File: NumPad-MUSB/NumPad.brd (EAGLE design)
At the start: 85.1 x 137.2 mm, 149 parts, among them J1 J, J10 J, J11 J, J12 J, J13 J, J14 J, J15 J, J16 J, J17 J, J2 J, J3 J, J4 J, J5 J, J6 J, J7 J, J8 J, J9 J

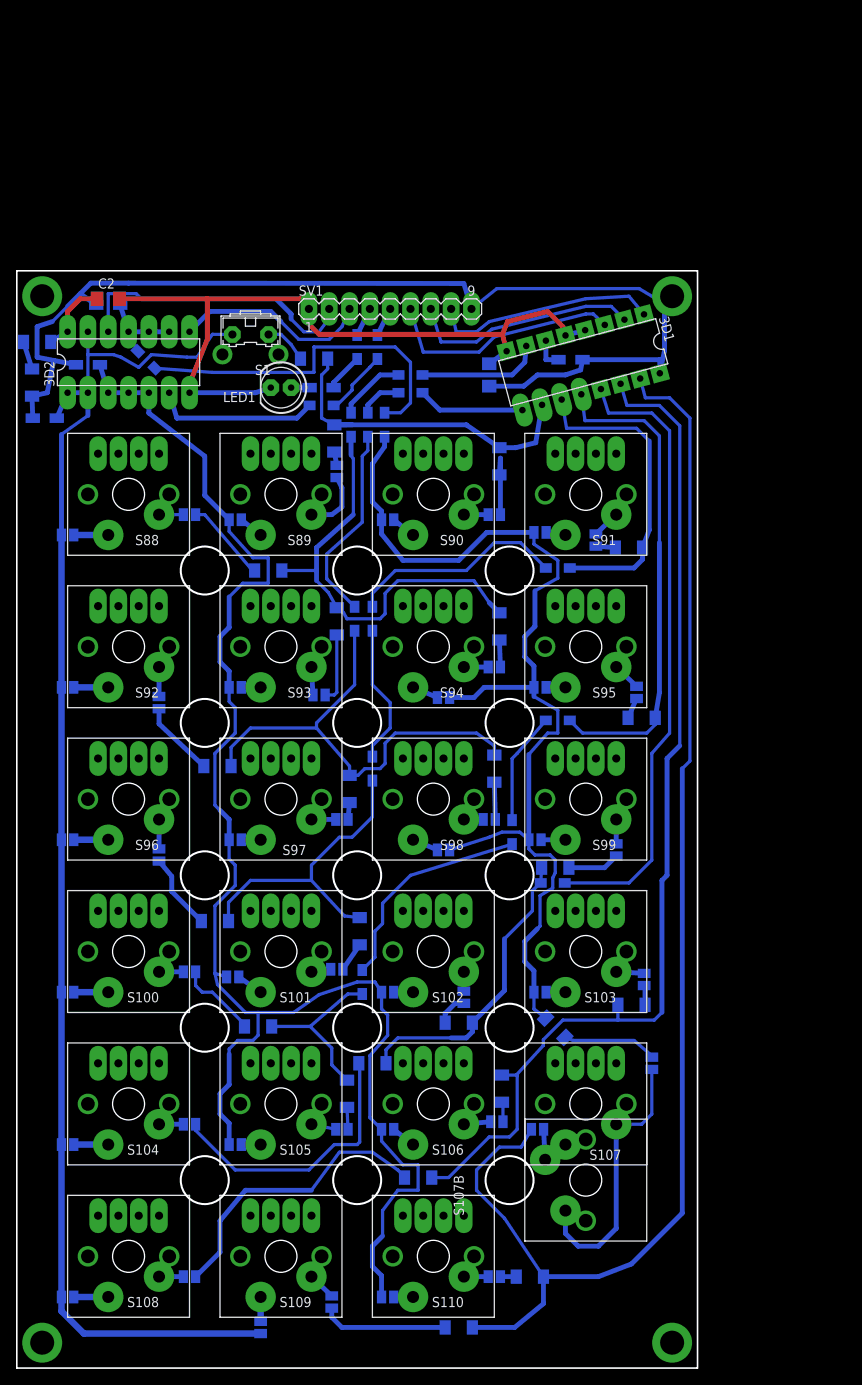
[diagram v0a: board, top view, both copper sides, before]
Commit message: err
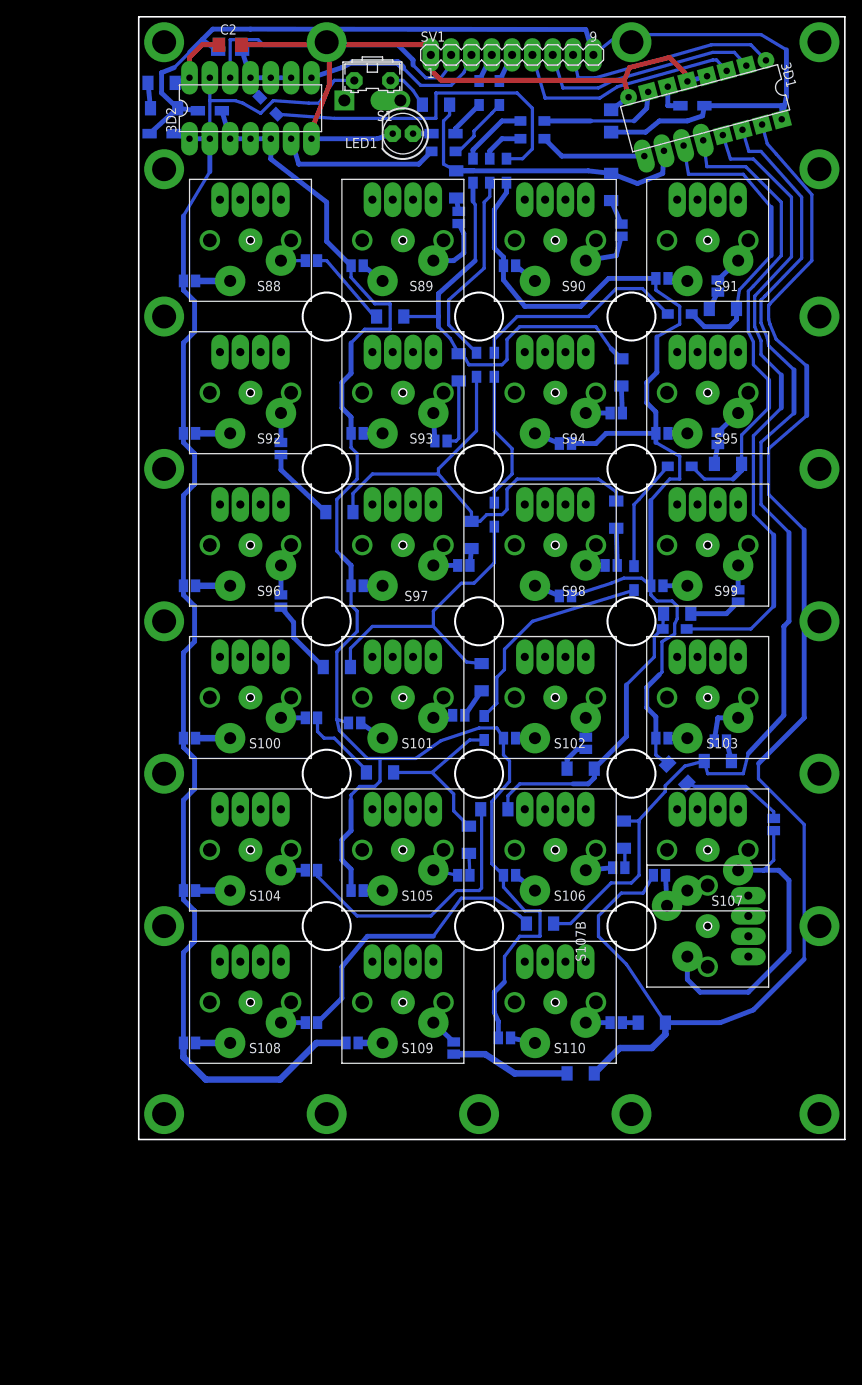
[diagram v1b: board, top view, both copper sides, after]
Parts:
- added U$1: (no value), kbmx:18X18
- S107B: device cherrymx:CHERRY-MX -> cherrymx:CHERRY-MX-4P
- moved JB90 38.9 mm to (78.7, 151.1), turned to 90 degrees
- moved R1 38.4 mm to (21.3, 163.2)
- moved D2 38.1 mm to (21.6, 166.4), turned to 180 degrees
- moved JA109 37.4 mm to (45.1, 49.5), turned to 0 degrees
- moved D90 37.0 mm to (77.5, 156.5)
- moved D1 35.9 mm to (21.3, 169.5)
- moved JA110 35.5 mm to (64.1, 50.2)
- moved JB91 35.2 mm to (90.8, 144.1)
- moved D88 35.2 mm to (49.8, 140.3)
- moved D93 35.2 mm to (58.4, 134.0)
- moved J11 35.2 mm to (60.6, 134.3)
- moved J12 35.2 mm to (62.3, 158.6)
- moved J6 35.2 mm to (62.9, 134.3)
- moved J8 35.2 mm to (64.4, 158.6)
- moved J9 35.2 mm to (60.2, 158.6)
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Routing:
- net SCK: track 168.1 -> 177.6 mm
- net N$277: track 9.16 -> 3.20 mm
- net +5V: track 137.7 -> 132.5 mm
- net N$319: track 34.4 -> 39.6 mm
- net N$278: track 3.05 -> 6.36 mm
- net N$11: track 78.3 -> 81.5 mm
- net N$36: track 130.4 -> 132.6 mm
- net N$35: track 61.3 -> 59.3 mm
- net N$317: track 3.50 -> 5.43 mm
- net N$33: track 42.7 -> 40.9 mm
- net N$14: track 176.8 -> 178.4 mm
- net N$3: track 11.8 -> 13.0 mm
- net N$34: track 39.1 -> 38.1 mm
- net N$7: track 190.9 -> 189.9 mm
- net COLN3: track 24.6 -> 23.7 mm
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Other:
- board size 85.1 x 137.2 mm -> 88.3 x 140.3 mm
